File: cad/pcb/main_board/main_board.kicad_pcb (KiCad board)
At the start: 2 copper layers, 70.5 x 56.5 mm, 76 parts, among them J1 USB_B_Micro, J2 Conn_ARM_JTAG_SWD_10, U1 STM32F401R_B-C_Tx, U2 TLV75533PDRVR, Y1 Crystal_GND23

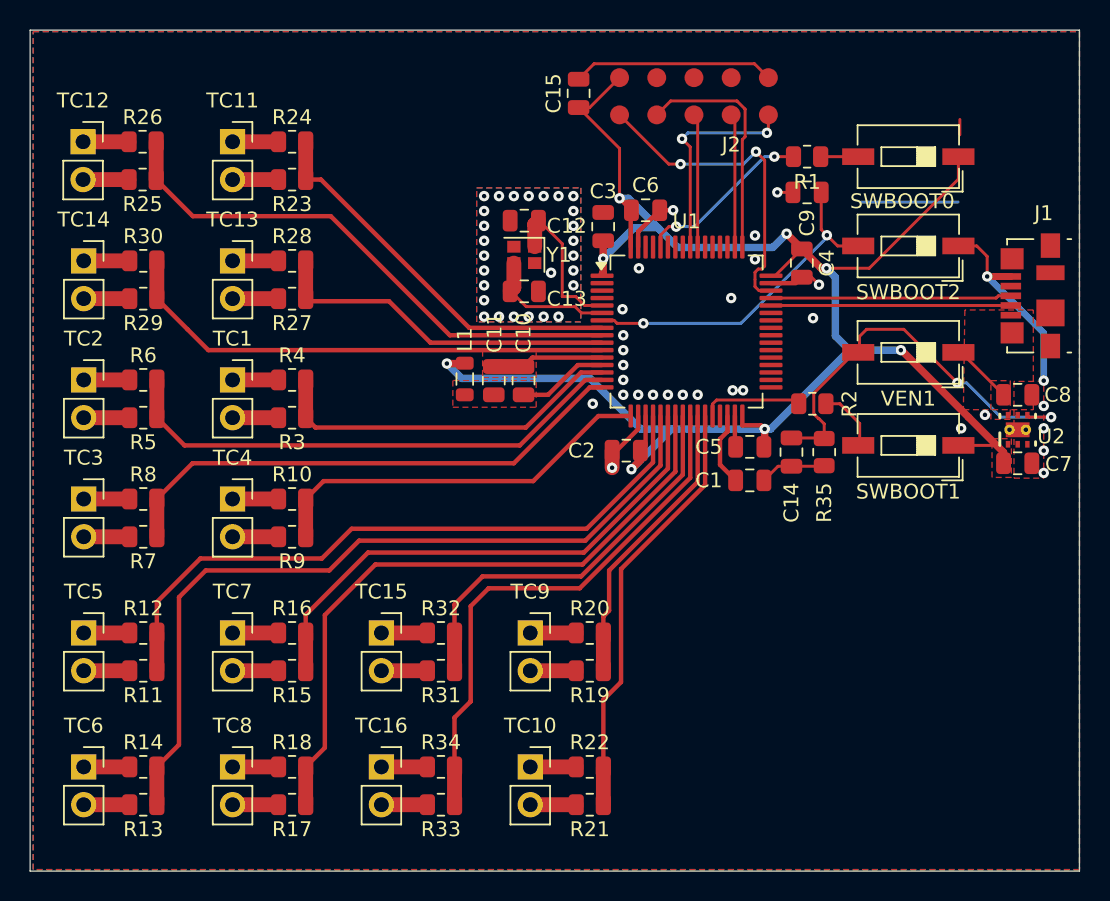
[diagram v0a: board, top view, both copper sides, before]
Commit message: It looks messy
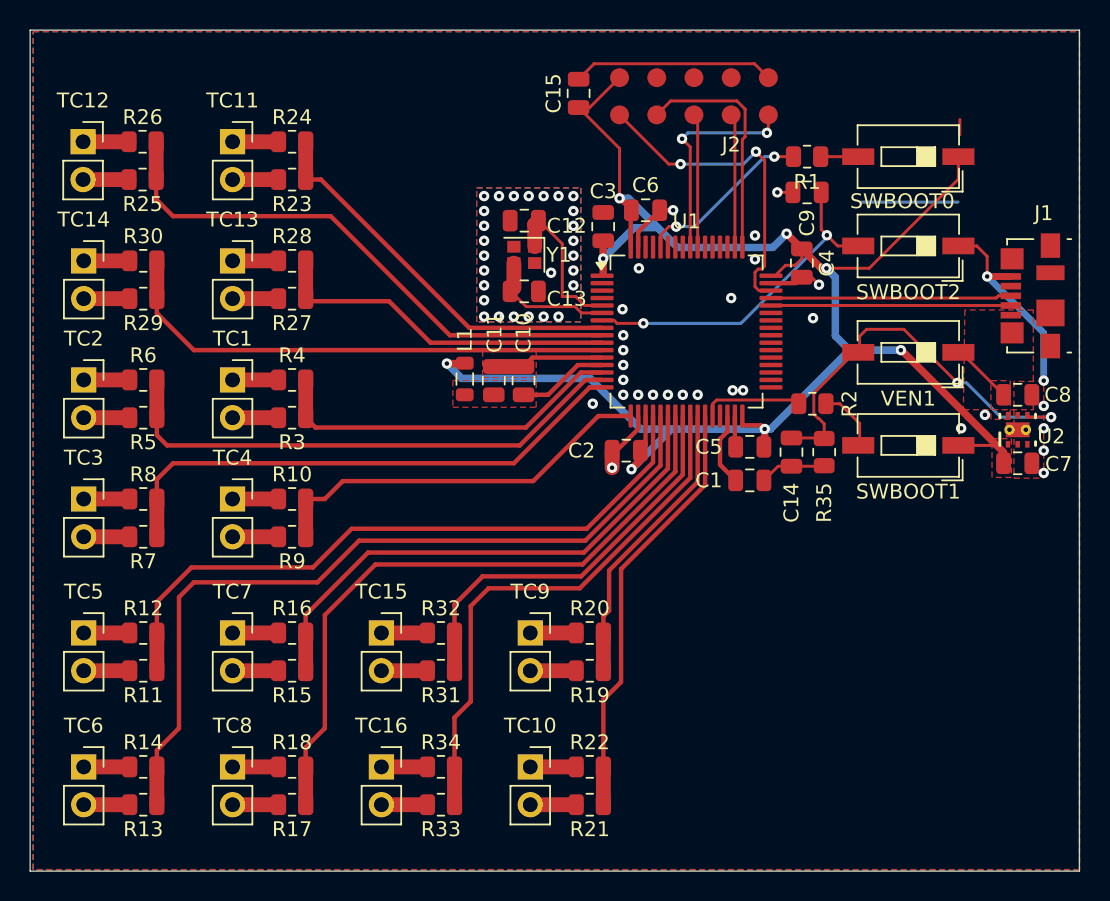
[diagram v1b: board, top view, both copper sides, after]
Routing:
- net /MCU/ADC_IN11: track 36.8 -> 37.6 mm
- net /MCU/ADC_IN2: track 35.6 -> 36.3 mm
- net /MCU/ADC_IN1: track 35.0 -> 35.7 mm
- net /MCU/ADC_IN13: track 33.9 -> 34.5 mm
